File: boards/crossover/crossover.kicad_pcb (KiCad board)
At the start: 2 copper layers, 56.6 x 33.3 mm, 29 parts, among them P1 CONN_01X07, P2 CONN_01X07, U1 TL074

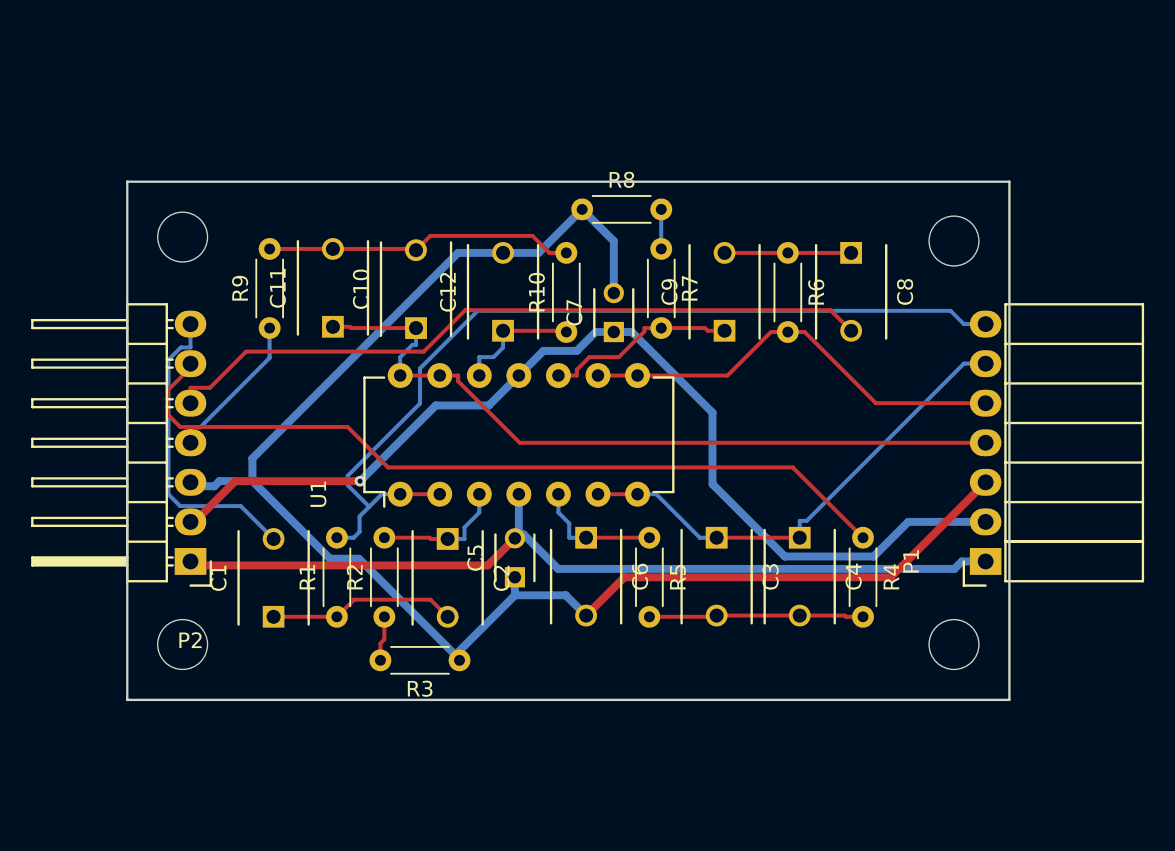
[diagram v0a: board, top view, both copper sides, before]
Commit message: more boards work
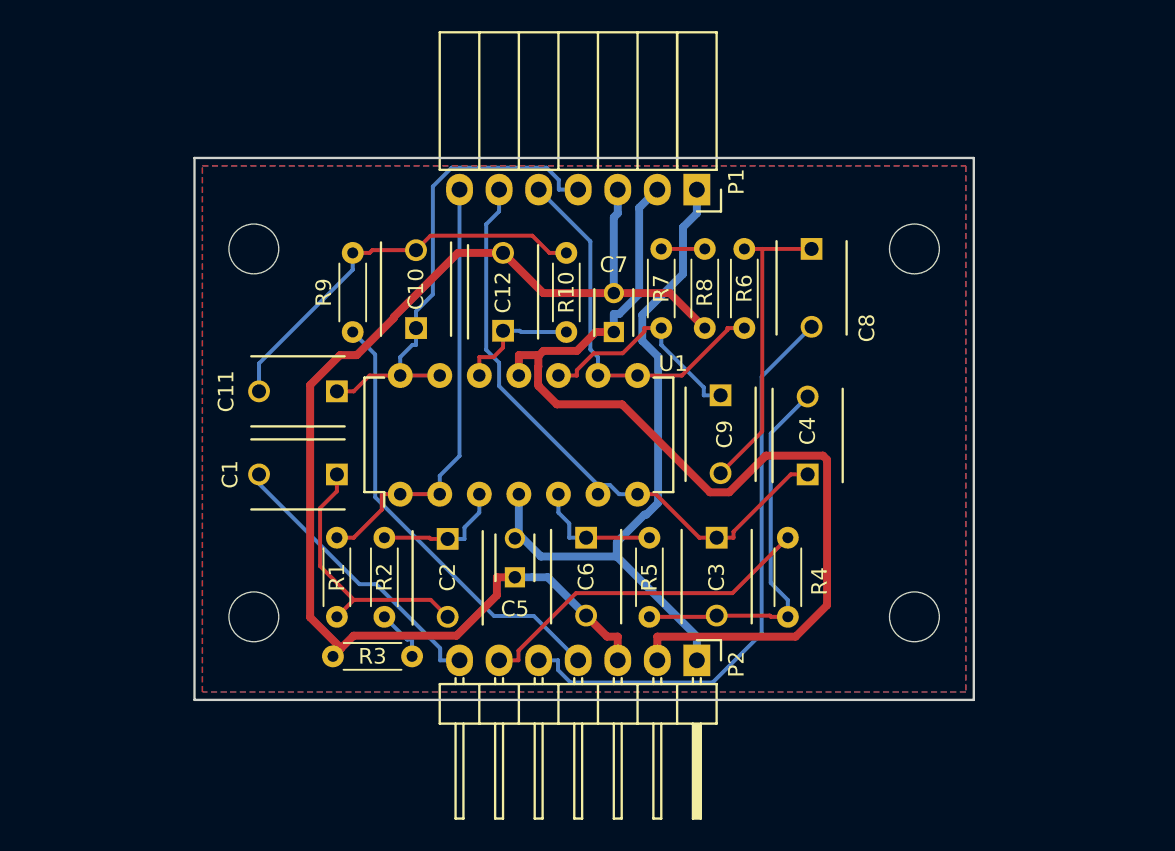
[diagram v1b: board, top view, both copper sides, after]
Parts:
- moved P2 33.1 mm to (154.2, 100.1), turned to 270 degrees
- moved P1 30.2 mm to (154.2, 69.8), turned to 180 degrees
- moved R8 11.0 mm to (154.7, 78.7), turned to 90 degrees
- moved C1 10.0 mm to (131.1, 88.1), turned to 180 degrees
- moved R3 8.13 mm to (130.8, 99.8), turned to 0 degrees
- moved R9 5.34 mm to (132.1, 79.0)
- moved mnt4 4.91 mm to (125.7, 97.3)
- moved R4 4.83 mm to (160.0, 92.2)
- moved mnt3 4.64 mm to (125.7, 73.7)
- moved C11 4.15 mm to (131.1, 82.8), turned to 180 degrees
- moved C9 4.15 mm to (155.7, 83.1), turned to 270 degrees
- moved C4 4.10 mm to (161.3, 88.1), turned to 90 degrees
- moved mnt2 3.10 mm to (168.1, 97.3)
- moved R6 2.81 mm to (157.2, 73.7)
- moved mnt1 2.59 mm to (168.1, 73.7)
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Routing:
- net /right_woofer_in: track 51.8 -> 22.2 mm
- net /right_high_out: track 57.9 -> 28.4 mm
- net GND: track 98.9 -> 79.5 mm
- net /left_woofer_in: track 10.1 -> 28.6 mm
- net /left_low_out: track 48.6 -> 30.9 mm
- net Net-(C8-Pad1): track 8.13 -> 19.8 mm
- net Net-(C3-Pad2): track 13.8 -> 24.5 mm
- net +15V: track 55.9 -> 45.2 mm
- net /left_tweeter_ph: track 46.3 -> 37.6 mm
- net /right_low_out: track 31.3 -> 39.6 mm
- net Net-(C10-Pad2): track 19.9 -> 26.0 mm
- net Net-(C1-Pad1): track 12.1 -> 17.4 mm
- net /left_high_out: track 27.9 -> 24.2 mm
- net Net-(C9-Pad1): track 12.4 -> 14.7 mm
- net /right_tweeter_ph: track 19.8 -> 18.6 mm
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- added copper zone on B.Cu, net GND
- added copper zone on F.Cu, net GND
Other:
- board size 56.6 x 33.3 mm -> 50 x 34.8 mm
